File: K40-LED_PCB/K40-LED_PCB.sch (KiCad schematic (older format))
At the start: 14 parts, among them p1 12V_Pad

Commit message: More Footprint updates
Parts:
- p1: footprint 12V_Pad:12V_Supply_Pad -> 12V_Through_Hole:12V_Through_Hole
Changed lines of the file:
@@
 F 0 "p1" V 7029 3053 50  0000 L CNN
 F 1 "12V_Pad" V 7120 3053 50  0000 L CNN
-F 2 "12V_Pad:12V_Supply_Pad" H 7075 3100 50  0001 C CNN
+F 2 "12V_Through_Hole:12V_Through_Hole" H 7075 3100 50  0001 C CNN
 F 3 "" H 7075 3100 50  0001 C CNN
 	1    7075 3100

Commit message: Footprint updates
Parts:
- D1, D10, D11, D12, D2, D3, D4, D5, D6, D7, D8, D9: footprint SPMWH1228FD5WATUS3_FOOTPRINT:LED_SPMWH1228FD5WARMSE -> Cree_MX3AWT-A1-R250-000BE3:Cree_MX3AWT-A1-R250-000BE3
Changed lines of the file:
@@
 F 0 "D4" H 4700 3831 50  0000 C CNN
 F 1 "LTST-C190KGKT" H 4700 3740 50  0000 C CNN
-F 2 "SPMWH1228FD5WATUS3_FOOTPRINT:LED_SPMWH1228FD5WARMSE" H 4750 3500 50  0001 L BNN
+F 2 "Cree_MX3AWT-A1-R250-000BE3:Cree_MX3AWT-A1-R250-000BE3" H 4750 3500 50  0001 L BNN
 F 3 "" H 4750 3500 50  0001 L BNN
 	1    4750 3500
@@
 F 0 "D7" H 4700 4531 50  0000 C CNN
 F 1 "LTST-C190KGKT" H 4700 4440 50  0000 C CNN
-F 2 "SPMWH1228FD5WATUS3_FOOTPRINT:LED_SPMWH1228FD5WARMSE" H 4750 4200 50  0001 L BNN
+F 2 "Cree_MX3AWT-A1-R250-000BE3:Cree_MX3AWT-A1-R250-000BE3" H 4750 4200 50  0001 L BNN
 F 3 "" H 4750 4200 50  0001 L BNN
 	1    4750 4200
@@
 F 0 "D10" H 6200 3131 50  0000 C CNN
 F 1 "LTST-C190KGKT" H 6200 3040 50  0000 C CNN
-F 2 "SPMWH1228FD5WATUS3_FOOTPRINT:LED_SPMWH1228FD5WARMSE" H 6250 2800 50  0001 L BNN
+F 2 "Cree_MX3AWT-A1-R250-000BE3:Cree_MX3AWT-A1-R250-000BE3" H 6250 2800 50  0001 L BNN
 F 3 "" H 6250 2800 50  0001 L BNN
 	1    6250 2800
@@
 F 0 "D2" H 5200 3131 50  0000 C CNN
 F 1 "LTST-C190KGKT" H 5200 3040 50  0000 C CNN
-F 2 "SPMWH1228FD5WATUS3_FOOTPRINT:LED_SPMWH1228FD5WARMSE" H 5250 2800 50  0001 L BNN
+F 2 "Cree_MX3AWT-A1-R250-000BE3:Cree_MX3AWT-A1-R250-000BE3" H 5250 2800 50  0001 L BNN
 F 3 "" H 5250 2800 50  0001 L BNN
 	1    5250 2800
@@
 F 0 "D5" H 5200 3831 50  0000 C CNN
 F 1 "LTST-C190KGKT" H 5200 3740 50  0000 C CNN
-F 2 "SPMWH1228FD5WATUS3_FOOTPRINT:LED_SPMWH1228FD5WARMSE" H 5250 3500 50  0001 L BNN
+F 2 "Cree_MX3AWT-A1-R250-000BE3:Cree_MX3AWT-A1-R250-000BE3" H 5250 3500 50  0001 L BNN
 F 3 "" H 5250 3500 50  0001 L BNN
 	1    5250 3500
@@
 F 0 "D8" H 5200 4531 50  0000 C CNN
 F 1 "LTST-C190KGKT" H 5200 4440 50  0000 C CNN
-F 2 "SPMWH1228FD5WATUS3_FOOTPRINT:LED_SPMWH1228FD5WARMSE" H 5250 4200 50  0001 L BNN
+F 2 "Cree_MX3AWT-A1-R250-000BE3:Cree_MX3AWT-A1-R250-000BE3" H 5250 4200 50  0001 L BNN
 F 3 "" H 5250 4200 50  0001 L BNN
 	1    5250 4200
@@
 F 0 "D11" H 6200 3831 50  0000 C CNN
 F 1 "LTST-C190KGKT" H 6200 3740 50  0000 C CNN
-F 2 "SPMWH1228FD5WATUS3_FOOTPRINT:LED_SPMWH1228FD5WARMSE" H 6250 3500 50  0001 L BNN
+F 2 "Cree_MX3AWT-A1-R250-000BE3:Cree_MX3AWT-A1-R250-000BE3" H 6250 3500 50  0001 L BNN
 F 3 "" H 6250 3500 50  0001 L BNN
 	1    6250 3500
@@
 F 0 "D3" H 5700 3131 50  0000 C CNN
 F 1 "LTST-C190KGKT" H 5700 3040 50  0000 C CNN
-F 2 "SPMWH1228FD5WATUS3_FOOTPRINT:LED_SPMWH1228FD5WARMSE" H 5750 2800 50  0001 L BNN
+F 2 "Cree_MX3AWT-A1-R250-000BE3:Cree_MX3AWT-A1-R250-000BE3" H 5750 2800 50  0001 L BNN
 F 3 "" H 5750 2800 50  0001 L BNN
 	1    5750 2800
@@
 F 0 "D6" H 5700 3831 50  0000 C CNN
 F 1 "LTST-C190KGKT" H 5700 3740 50  0000 C CNN
-F 2 "SPMWH1228FD5WATUS3_FOOTPRINT:LED_SPMWH1228FD5WARMSE" H 5750 3500 50  0001 L BNN
+F 2 "Cree_MX3AWT-A1-R250-000BE3:Cree_MX3AWT-A1-R250-000BE3" H 5750 3500 50  0001 L BNN
 F 3 "" H 5750 3500 50  0001 L BNN
 	1    5750 3500
@@
 F 0 "D9" H 5700 4531 50  0000 C CNN
 F 1 "LTST-C190KGKT" H 5700 4440 50  0000 C CNN
-F 2 "SPMWH1228FD5WATUS3_FOOTPRINT:LED_SPMWH1228FD5WARMSE" H 5750 4200 50  0001 L BNN
+F 2 "Cree_MX3AWT-A1-R250-000BE3:Cree_MX3AWT-A1-R250-000BE3" H 5750 4200 50  0001 L BNN
 F 3 "" H 5750 4200 50  0001 L BNN
 	1    5750 4200
@@
 F 0 "D12" H 6200 4531 50  0000 C CNN
 F 1 "LTST-C190KGKT" H 6200 4440 50  0000 C CNN
-F 2 "SPMWH1228FD5WATUS3_FOOTPRINT:LED_SPMWH1228FD5WARMSE" H 6250 4200 50  0001 L BNN
+F 2 "Cree_MX3AWT-A1-R250-000BE3:Cree_MX3AWT-A1-R250-000BE3" H 6250 4200 50  0001 L BNN
 F 3 "" H 6250 4200 50  0001 L BNN
 	1    6250 4200
@@
 F 0 "D1" H 4700 3131 50  0000 C CNN
 F 1 "LTST-C190KGKT" H 4700 3040 50  0000 C CNN
-F 2 "SPMWH1228FD5WATUS3_FOOTPRINT:LED_SPMWH1228FD5WARMSE" H 4750 2800 50  0001 L BNN
+F 2 "Cree_MX3AWT-A1-R250-000BE3:Cree_MX3AWT-A1-R250-000BE3" H 4750 2800 50  0001 L BNN
 F 3 "" H 4750 2800 50  0001 L BNN
 	1    4750 2800

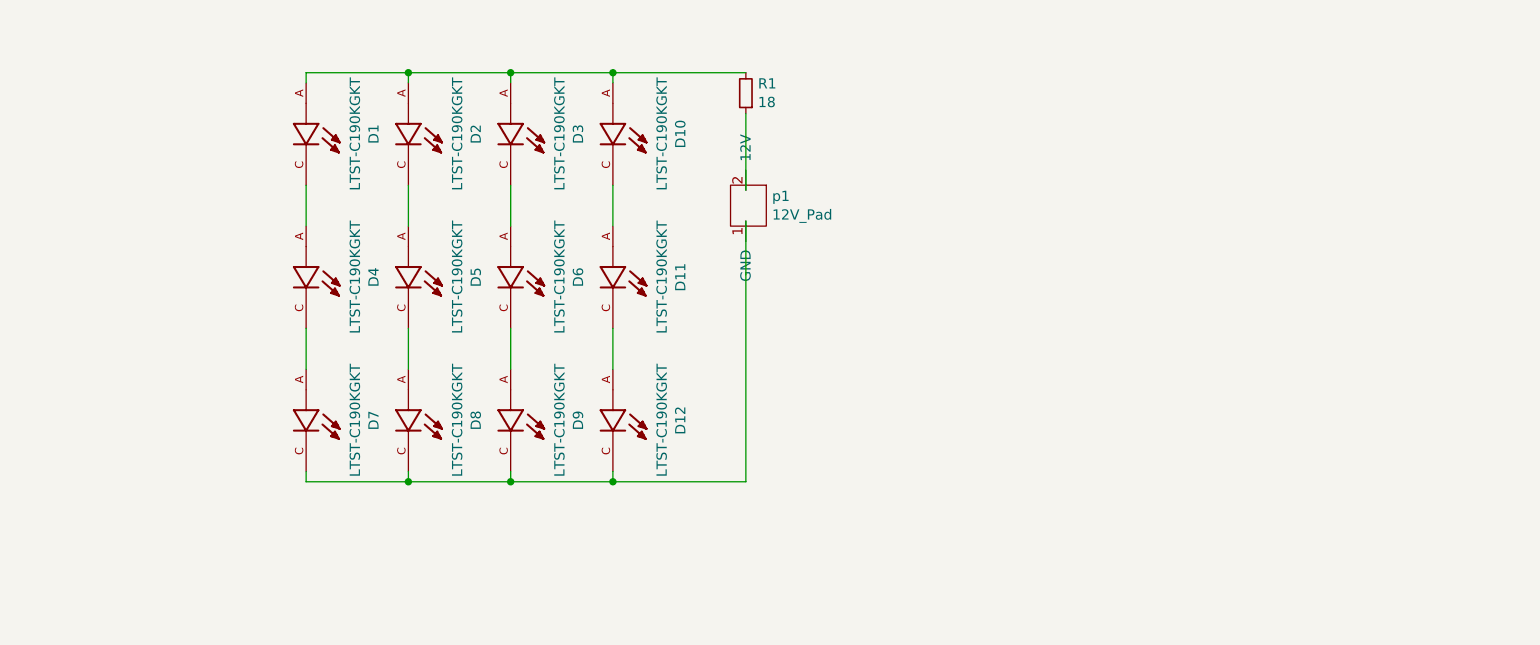
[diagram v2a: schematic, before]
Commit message: Major  PCB  Changes
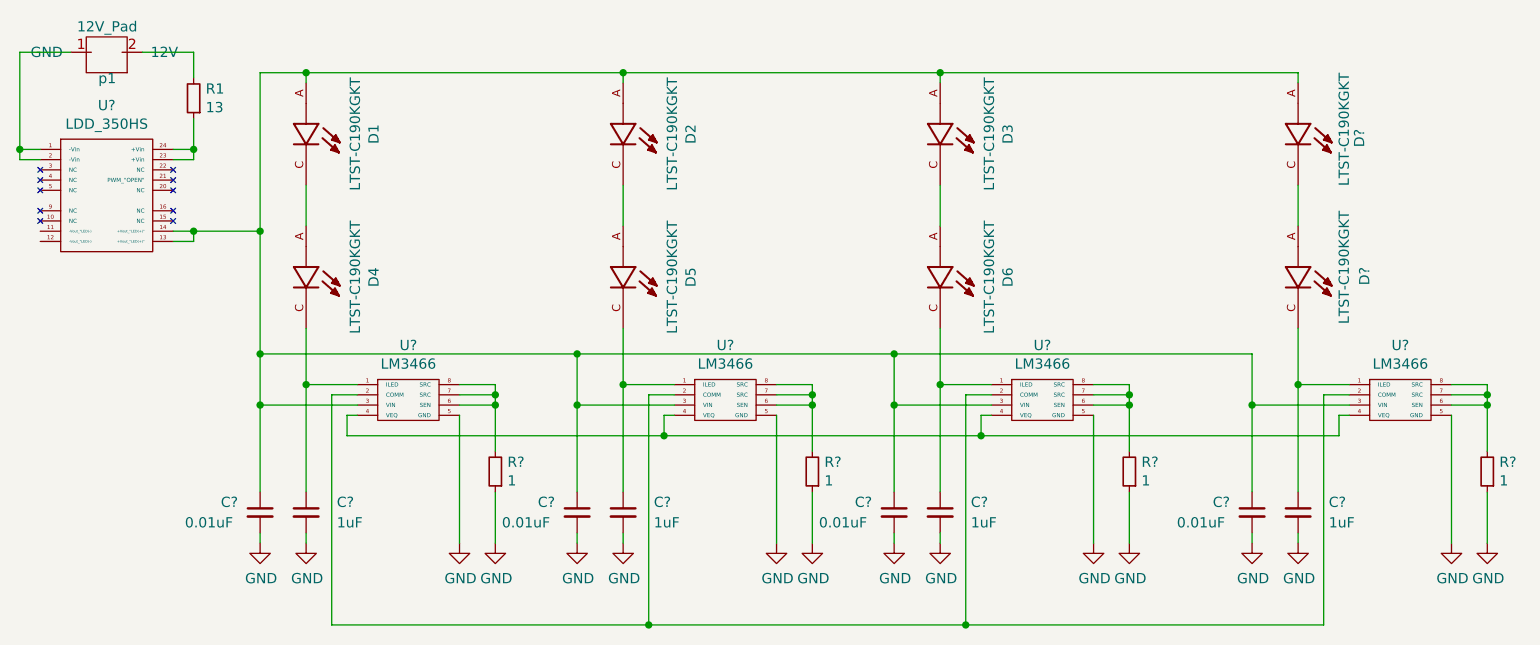
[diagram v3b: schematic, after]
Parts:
- removed D10, D11, D12, D7, D8, D9: LTST-C190KGKT, Cree_MX3AWT-A1-R250-000BE3:Cree_MX3AWT-A1-R250-000BE3, symbol LTST-C190KGKT:LTST-C190KGKT
- added C? (x4): 0.01uF, symbol Device:C_Small
- added C? (x4): 1uF, symbol Device:C_Small
- added D? (x2): LTST-C190KGKT, LEDC1608X35N, symbol LTST-C190KGKT:LTST-C190KGKT
- added R? (x4): 1, Resistor_SMD:R_0805_2012Metric, symbol Device:R_Small
- added U?: LDD_350HS, symbol LDD-350HS_SYMBOL:LDD_350HS
- added U? (x4): LM3466, symbol LM3466_SYMBOL:LM3466
- R1: value 18 -> 13
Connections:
- net at D1.A, D2.A, D3.A: now also C?.1, C?.1, C?.1, C?.1, D?.A, U?.13 (+Vout_"LED(+)"), U?.14 (+Vout_"LED(+)"), U?.3 (VIN), U?.3 (VIN), U?.3 (VIN), U?.3 (VIN); no longer R1.2
- net at D4.C: now also C?.1, U?.1 (ILED)
- net at D5.C: now also C?.1, U?.1 (ILED)
- net at D6.C: now also C?.1, U?.1 (ILED)
- net at p1.2 (12V): no longer R1.1
- new net: R1.1, U?.23 (+Vin), U?.24 (+Vin)
- new net: U?.1 (-Vin), U?.2 (-Vin)
- new net: U?.2 (COMM), U?.2 (COMM), U?.2 (COMM), U?.2 (COMM)
- new net: U?.4 (VEQ), U?.4 (VEQ), U?.4 (VEQ), U?.4 (VEQ)
- new net: R?.2, U?.6 (SEN), U?.7 (SRC), U?.8 (SRC) (x4)
- new net: D?.A, D?.C
- new net: C?.1, D?.C, U?.1 (ILED)
- new net GND: C?.2, C?.2, C?.2, C?.2, C?.2, C?.2, C?.2, C?.2, R?.1, R?.1, R?.1, R?.1, U?.5 (GND), U?.5 (GND), U?.5 (GND), U?.5 (GND)
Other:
- moved on the sheet: D2, D3, D5, D6, R1, p1
